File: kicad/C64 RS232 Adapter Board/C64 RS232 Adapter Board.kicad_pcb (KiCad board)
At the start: 2 copper layers, 63.6 x 56.9 mm, 31 parts, among them J1 RS232_HDR, J2 DB25_RS232, J3 C64_USER_PORT, J4 User Port Breakout, SW1 RESET, U1 MAX3241ECAI+T

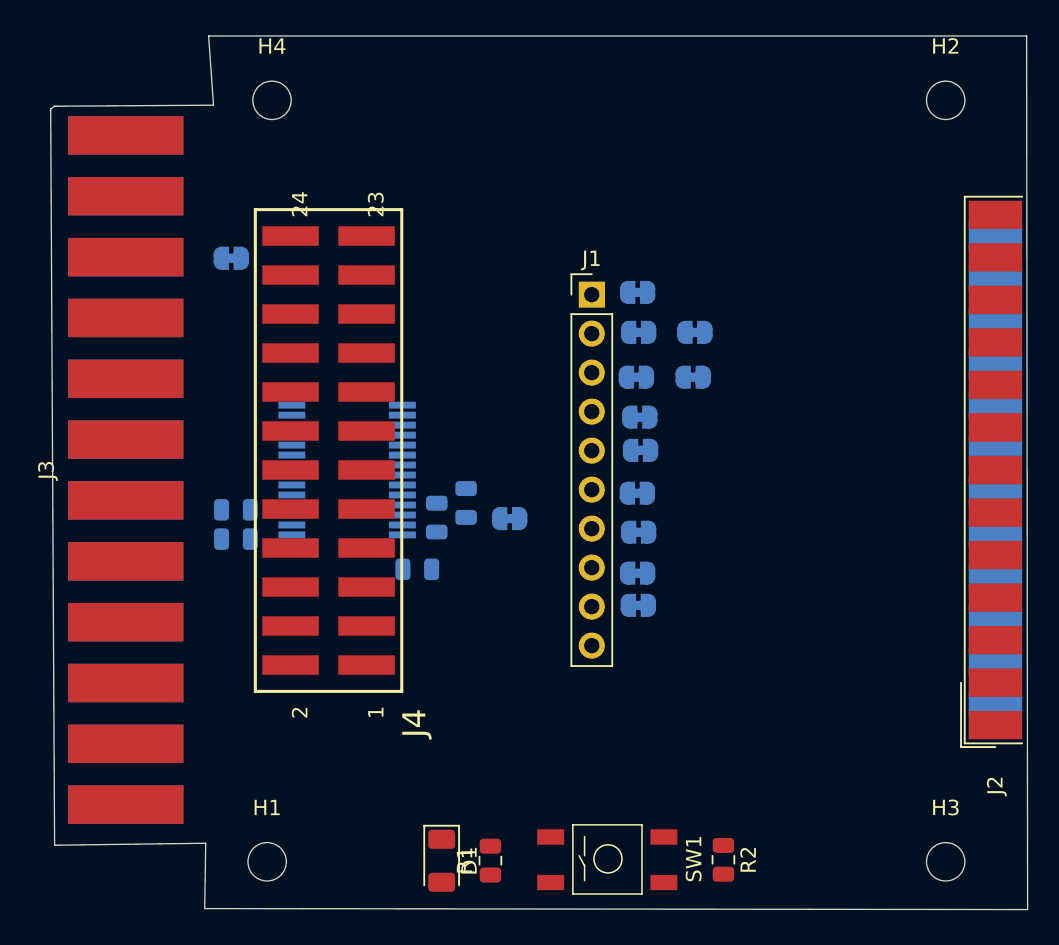
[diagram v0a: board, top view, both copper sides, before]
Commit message: before first routing attempt
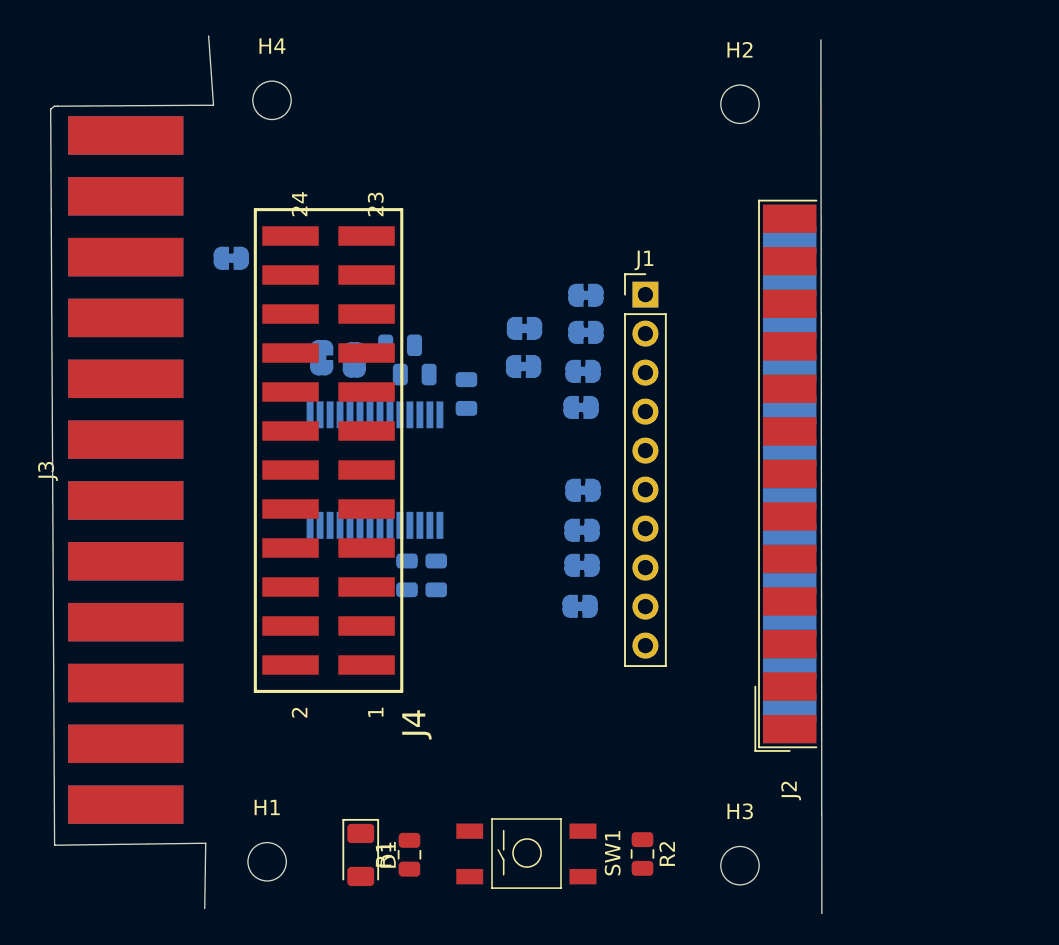
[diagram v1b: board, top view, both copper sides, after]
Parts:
- moved JP12 21.6 mm to (61.0, 72.6), turned to 270 degrees
- moved JP13 14.5 mm to (63.1, 72.8), turned to 270 degrees
- moved H2 13.4 mm to (88.2, 56.1)
- moved H3 13.4 mm to (88.2, 105.7)
- moved J2 13.4 mm to (91.4, 80.2)
- moved C2 13.3 mm to (68.4, 86.8), turned to 270 degrees
- moved C4 11.9 mm to (66.5, 86.8), turned to 90 degrees
- moved C3 11.9 mm to (70.4, 75.0), turned to 270 degrees
- moved C5 11.1 mm to (66.1, 71.8), turned to 0 degrees
- moved JP1 11.1 mm to (74.2, 70.7), turned to 0 degrees
- moved JP8 11.1 mm to (74.1, 73.2), turned to 180 degrees
- moved C1 9.43 mm to (67.0, 73.7), turned to 0 degrees
- moved D1 5.28 mm to (63.5, 105.0)
- moved R1 5.28 mm to (66.7, 105.0)
- moved R2 5.28 mm to (81.9, 105.0)
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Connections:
- C1 pad 1: Net-(C1-Pad1) -> (no net)
- C1 pad 2: Net-(C1-Pad2) -> (no net)
- C2 pad 1: Net-(C2-Pad1) -> (no net)
- C2 pad 2: Net-(C2-Pad2) -> (no net)
- C3 pad 1: GND -> (no net)
- C3 pad 2: Net-(C3-Pad2) -> (no net)
- C4 pad 1: GND -> (no net)
- C4 pad 2: Net-(C4-Pad2) -> (no net)
- C5 pad 1: GND -> (no net)
- C5 pad 2: +5V -> (no net)
- JP13 pad 1: Net-(JP13-Pad1) -> (no net)
- JP13 pad 2: +5V -> (no net)
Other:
- board size 63.6 x 56.9 mm -> 50.2 x 57.1 mm
